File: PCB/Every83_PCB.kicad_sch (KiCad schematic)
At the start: 51 parts, among them J1 781710004, J3 Conn_01x02_Socket, J4 Conn_01x03_Pin, J6 Conn_01x02_Pin, J7 Conn_02x03_Counter_Clockwise, Q1 MMDT2222A, Q2 DMN24H3D5L, Q4 DMN24H3D5L, Q5 DMN24H3D5L, Q6 DMN24H3D5L, Q7 DMN24H3D5L, Q8 DMN24H3D5L, Q9 2N7002, SW101 KMR2, SW102 KMR2, U1 Core52840, U4 LDL40PU33RY, U6 BQ24075RGT

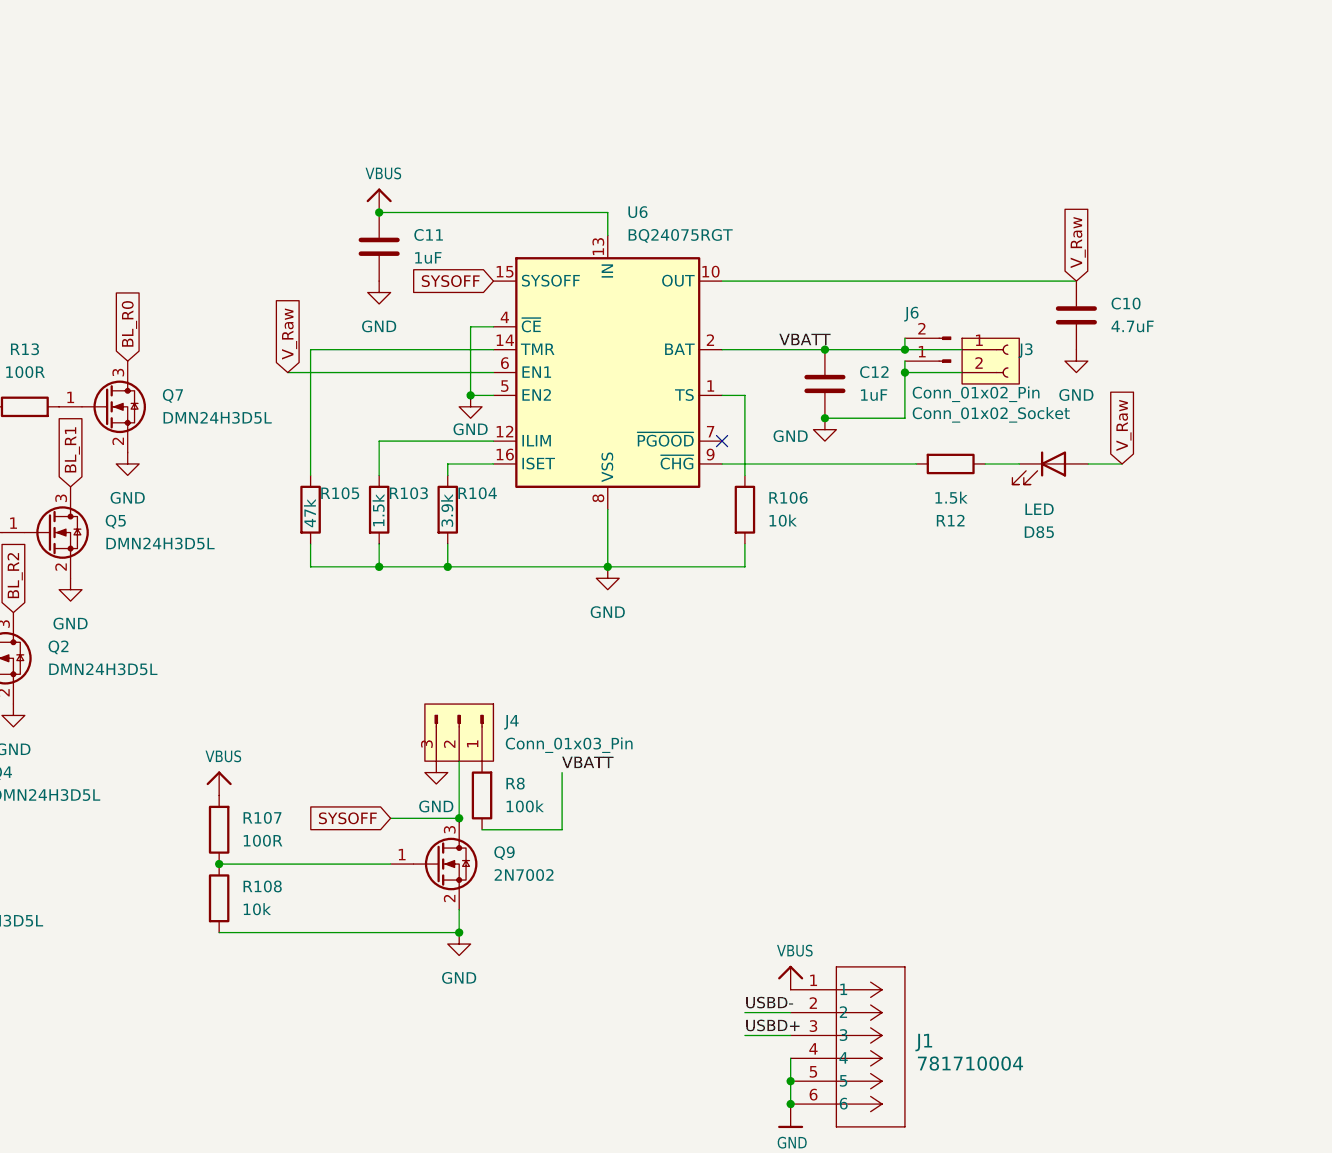
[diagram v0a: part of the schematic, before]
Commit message: Orginizing and small work done
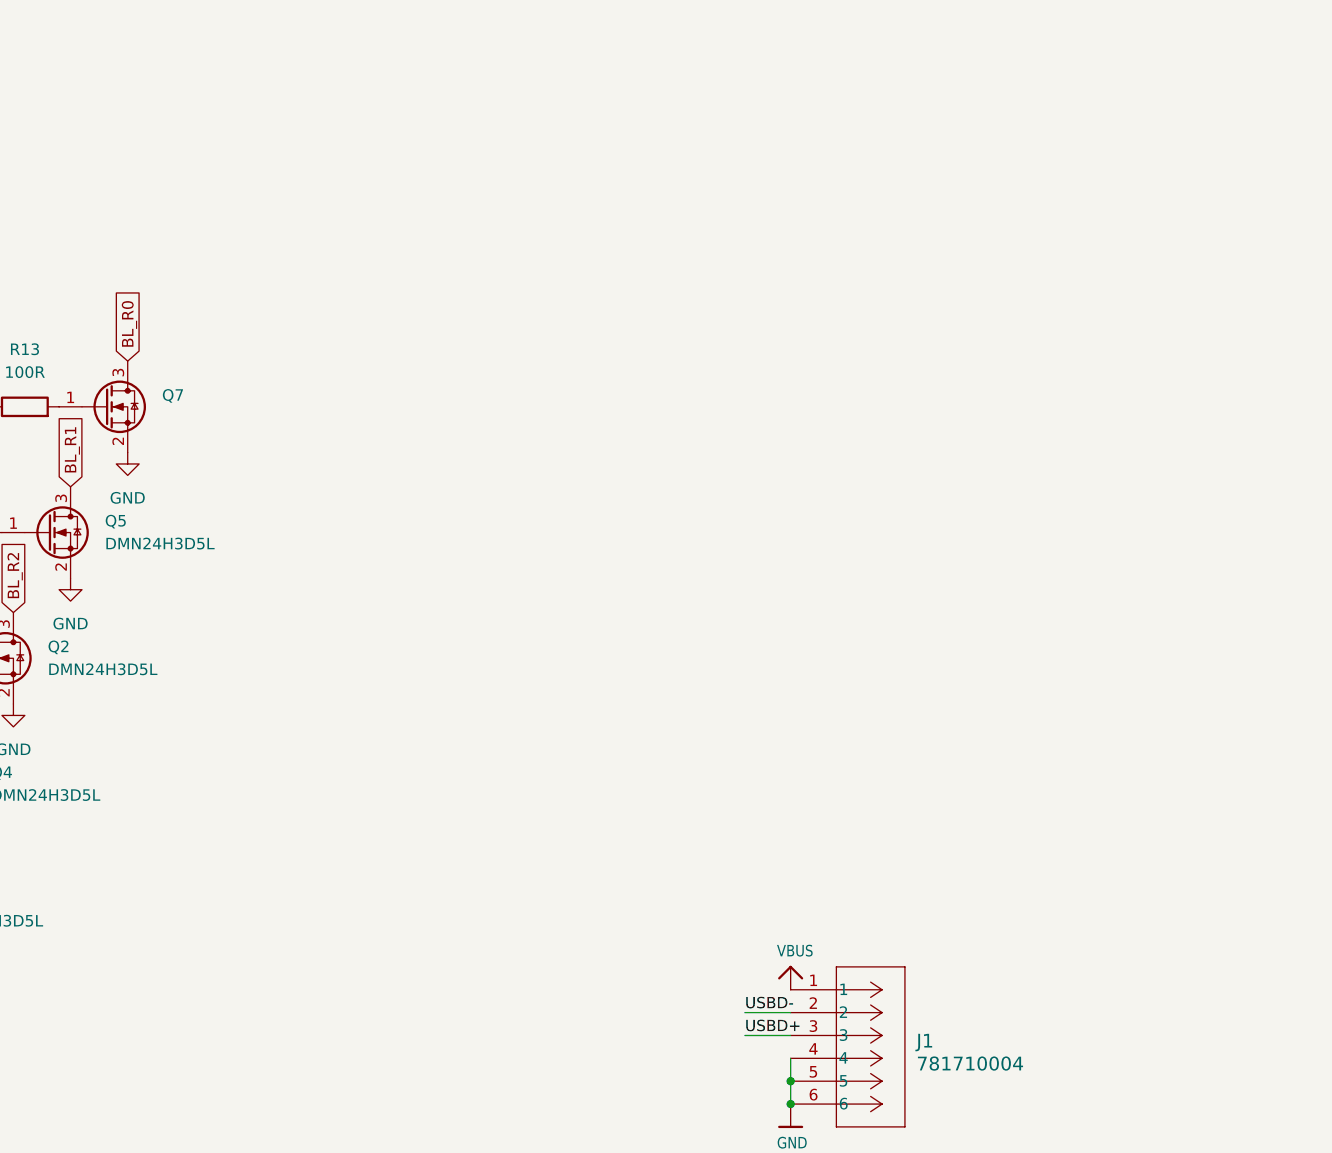
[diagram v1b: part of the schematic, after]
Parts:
- removed C10: 4.7uF, Capacitor_SMD:C_0402_1005Metric, symbol Device:C
- removed C11, C12: 1uF, Capacitor_SMD:C_0402_1005Metric, symbol Device:C
- removed D85: LED, JohnDeereLibrary:LED_WURTH_155060AS75300, symbol Device:LED
- removed J3: Conn_01x02_Socket, Connector_PinHeader_2.54mm:PinHeader_1x02_P2.54mm_Vertical, symbol Connector:Conn_01x02_Socket
- removed J4: Conn_01x03_Pin, Connector_Molex:Molex_Pico-EZmate_78171-0003_1x03-1MP_P1.20mm_Vertical, symbol Connector:Conn_01x03_Pin
- removed J6: Conn_01x02_Pin, Connector_Molex:Molex_Pico-EZmate_78171-0002_1x02-1MP_P1.20mm_Vertical, symbol Connector:Conn_01x02_Pin
- removed Q9: 2N7002, Package_TO_SOT_SMD:SOT-23, symbol Transistor_FET:2N7002
- removed R103, R12: 1.5k, Resistor_SMD:R_0402_1005Metric, symbol Device:R
- removed R104: 3.9k, Resistor_SMD:R_0402_1005Metric, symbol Device:R
- removed R105: 47k, Resistor_SMD:R_0402_1005Metric, symbol Device:R
- removed R106, R108: 10k, Resistor_SMD:R_0402_1005Metric, symbol Device:R
- removed R107: 100R, Resistor_SMD:R_0402_1005Metric, symbol Device:R
- removed R8: 100k, Resistor_SMD:R_0402_1005Metric, symbol Device:R
- removed U6: BQ24075RGT, Package_DFN_QFN:VQFN-16-1EP_3x3mm_P0.5mm_EP1.6x1.6mm, symbol Battery_Management:BQ24075RGT
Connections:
- no-connect marks 2 -> 1
